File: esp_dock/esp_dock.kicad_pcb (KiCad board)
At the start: 2 copper layers, 26.7 x 35.6 mm, 10 parts, among them P1 POWER, P2 LIGHT, P3 ESP, P4 SERIAL, P5 Pgrm, SW1 Switch_SPDT_x2, U1 LM3671

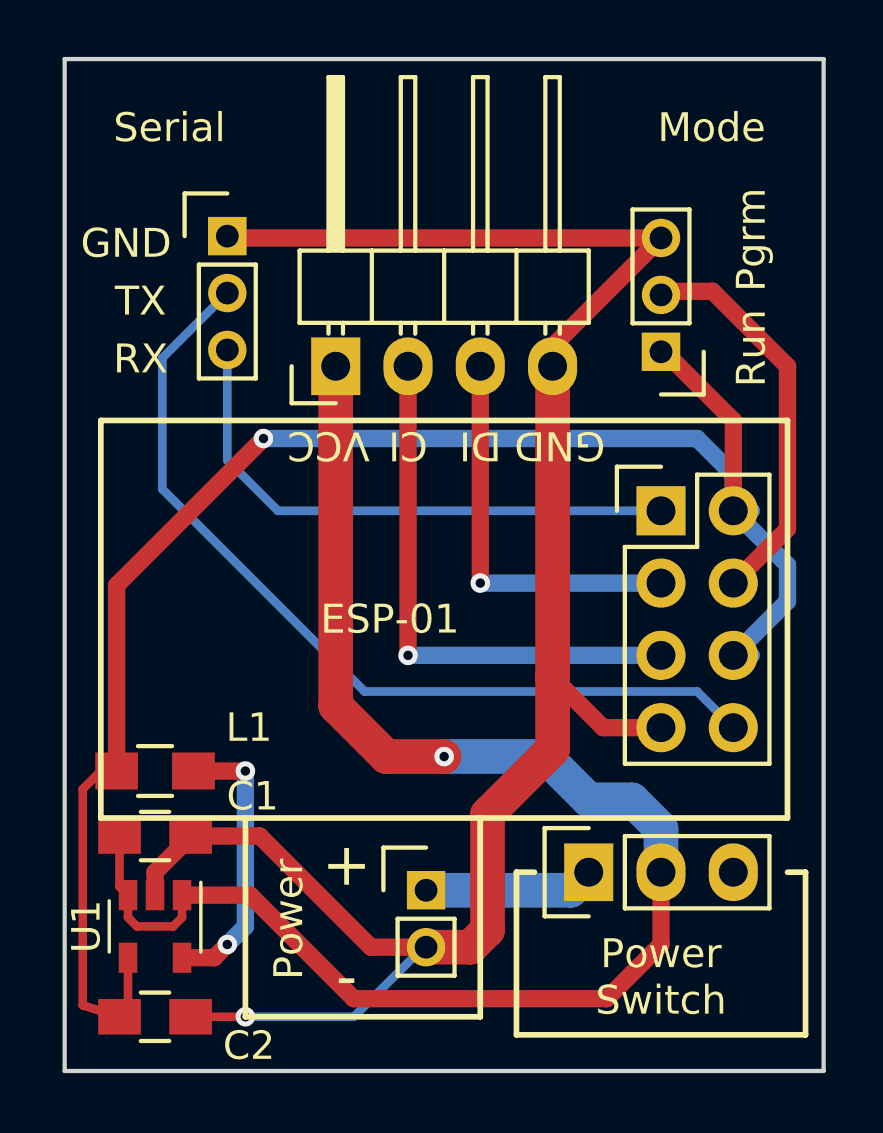
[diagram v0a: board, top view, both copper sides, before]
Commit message: Finished v1.5 of the board
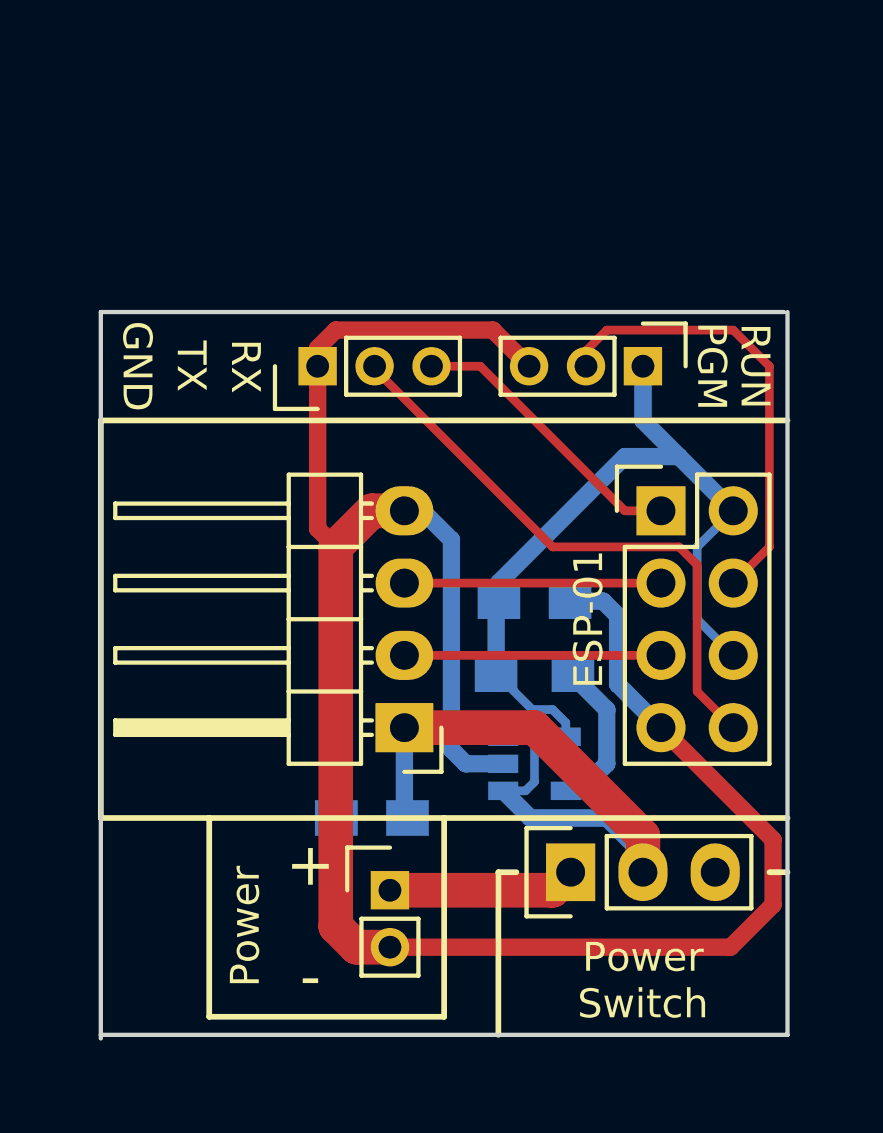
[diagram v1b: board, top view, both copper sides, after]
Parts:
- C1, C2, L1, U1: moved to B.Cu
- moved C2 19.8 mm to (142.9, 140.3)
- moved U1 14.5 mm to (142.9, 146.1), turned to 0 degrees
- moved L1 13.8 mm to (142.9, 142.9)
- moved P2 12.9 mm to (138.3, 144.8), turned to 180 degrees
- moved C1 7.65 mm to (137.2, 148.0), turned to 180 degrees
- moved P4 5.57 mm to (135.3, 132.1), turned to 90 degrees
- moved P1 1.27 mm to (137.8, 150.5)
- moved P5 0.81 mm to (146.7, 132.1), turned to 270 degrees
- moved SW1 0.63 mm to (144.1, 149.9)
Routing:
- net Net-(C2-Pad1): track 59.4 -> 27.7 mm, vias 1 -> 0
- net Net-(C1-Pad1): track 54.3 -> 25.1 mm, vias 1 -> 0
- net Net-(P3-Pad8): track 31.5 -> 20.5 mm
- net Net-(P2-Pad2): track 19.0 -> 9.02 mm, vias 1 -> 0
- net Net-(P3-Pad1): track 19.9 -> 10.2 mm
- net Net-(C1-Pad2): track 70.8 -> 79.8 mm, vias 1 -> 0
- net Net-(P2-Pad3): track 14.0 -> 9.02 mm, vias 1 -> 0
- net Net-(L1-Pad1): track 9.97 -> 5.64 mm, vias 2 -> 0
- net Net-(P3-Pad4): track 13.9 -> 16.0 mm
- net Net-(P1-Pad1): track 5.98 -> 6.61 mm
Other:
- board size 26.7 x 35.6 mm -> 24.1 x 25.5 mm
- board text added: "PGM"
- board text added: "RUN"
- board text added: "Raver Lights Endpoint v1.5 Copyright Bryan Hughes 2016"
- board text removed: "Mode"
- board text removed: "Pgrm"
- board text removed: "Raver Endpoint v1.0 Copyright (c) Bryan Hughes"
- board text removed: "Run"
- board text removed: "Serial"
